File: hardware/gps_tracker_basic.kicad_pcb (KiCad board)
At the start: 2 copper layers, 54 x 54 mm, 109 parts, among them J1 Conn_01x05, J2 USB_B_Micro, J3 Battery, J4 Conn_01x05, Q1 S8050, Q2 S8050, Q3 Si2301CDS, Q4 S8050, SW1 SW_Push_DPDT, SW2 SW_Push_DPDT, U1 STM32F030R8Tx, U10 L80-RE, U2 CAT24C256, U3 FT230XS, U4 UP501B, U5 USBLC6, U6 SIM800L, U7 MCP73812T-420I-OT, U8 TPS63020, U9 LP5907MFX-3.3, Y1 8 MHz

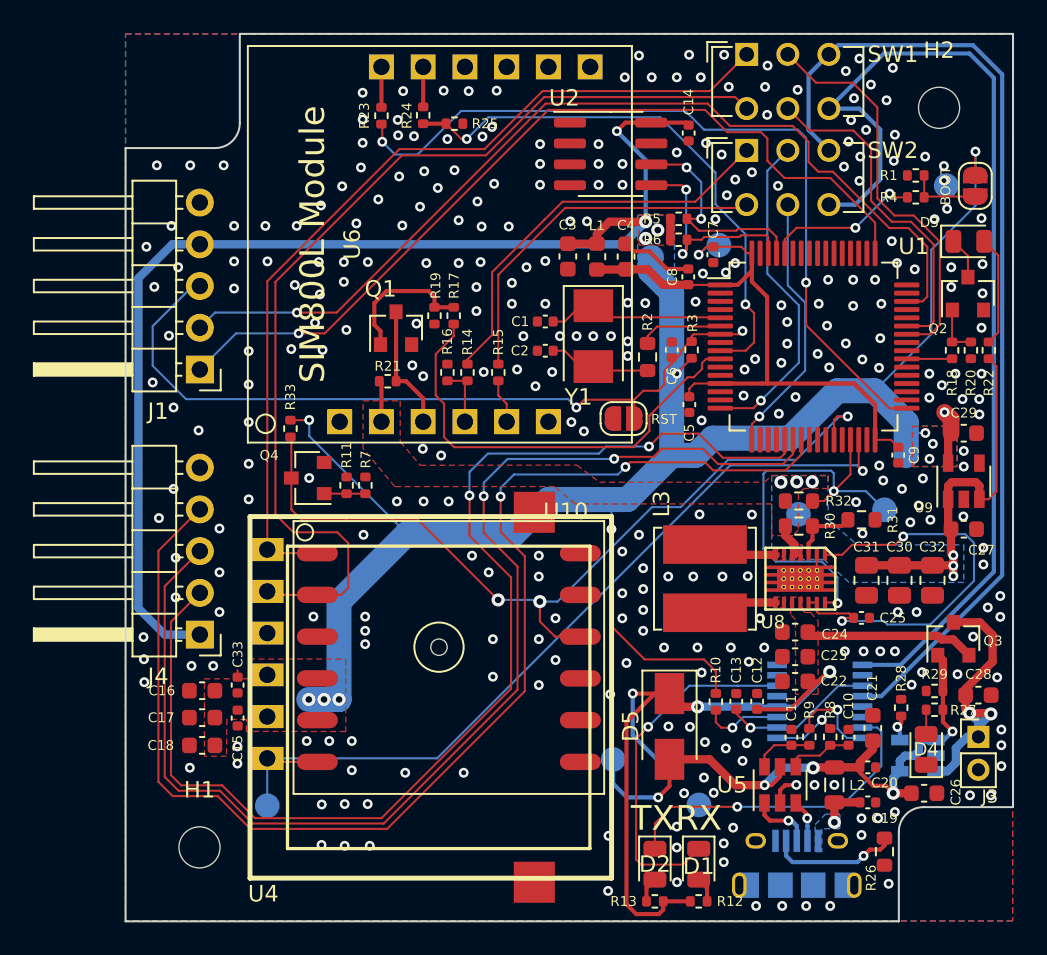
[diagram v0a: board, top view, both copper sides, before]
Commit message: Update kicad sheets
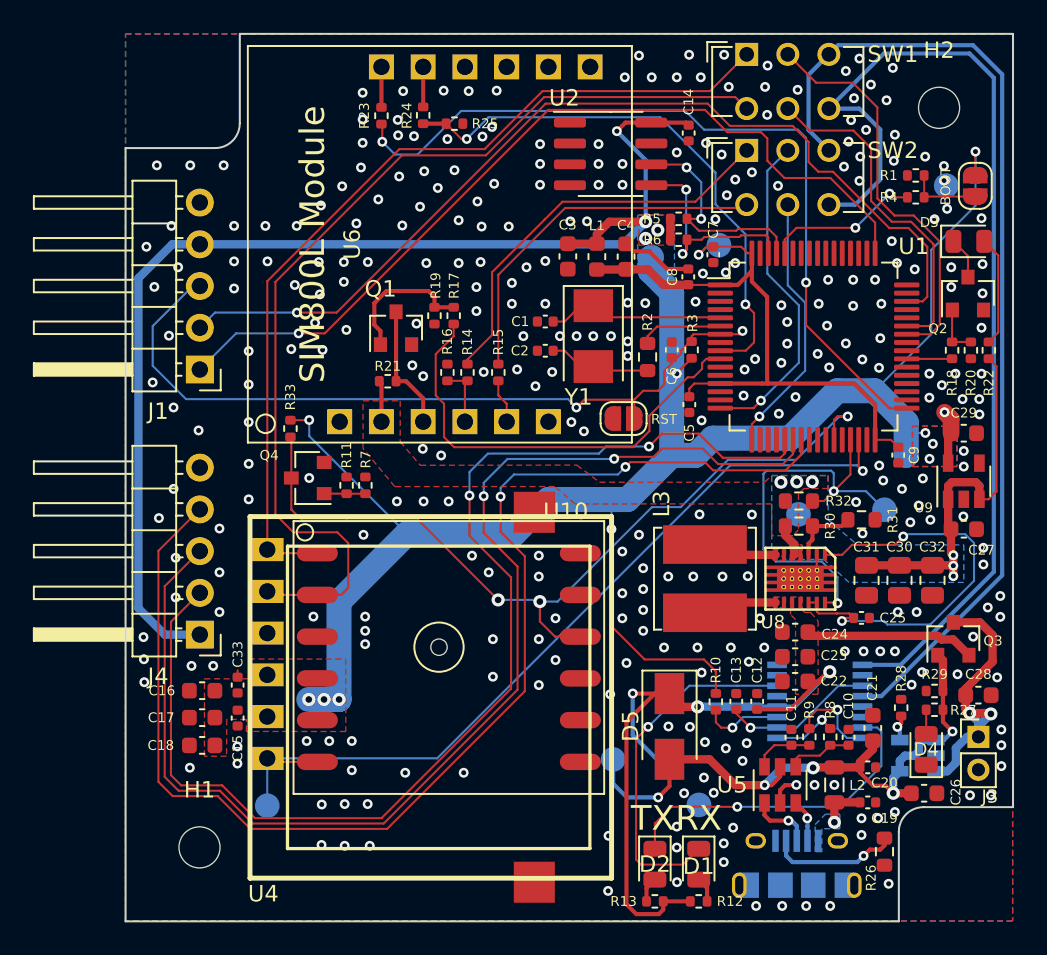
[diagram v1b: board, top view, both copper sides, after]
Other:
- net class Default removed
